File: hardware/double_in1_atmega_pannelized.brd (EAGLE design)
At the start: 82 x 70 mm, 76 parts, among them IC1 MEGA8-AI, IC2 MEGA8-AI, J1 AVR-ISP-6PINAVR-ISP-6PIN-SMAL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, J2 AVR-ISP-6PINAVR-ISP-6PIN-SMAL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

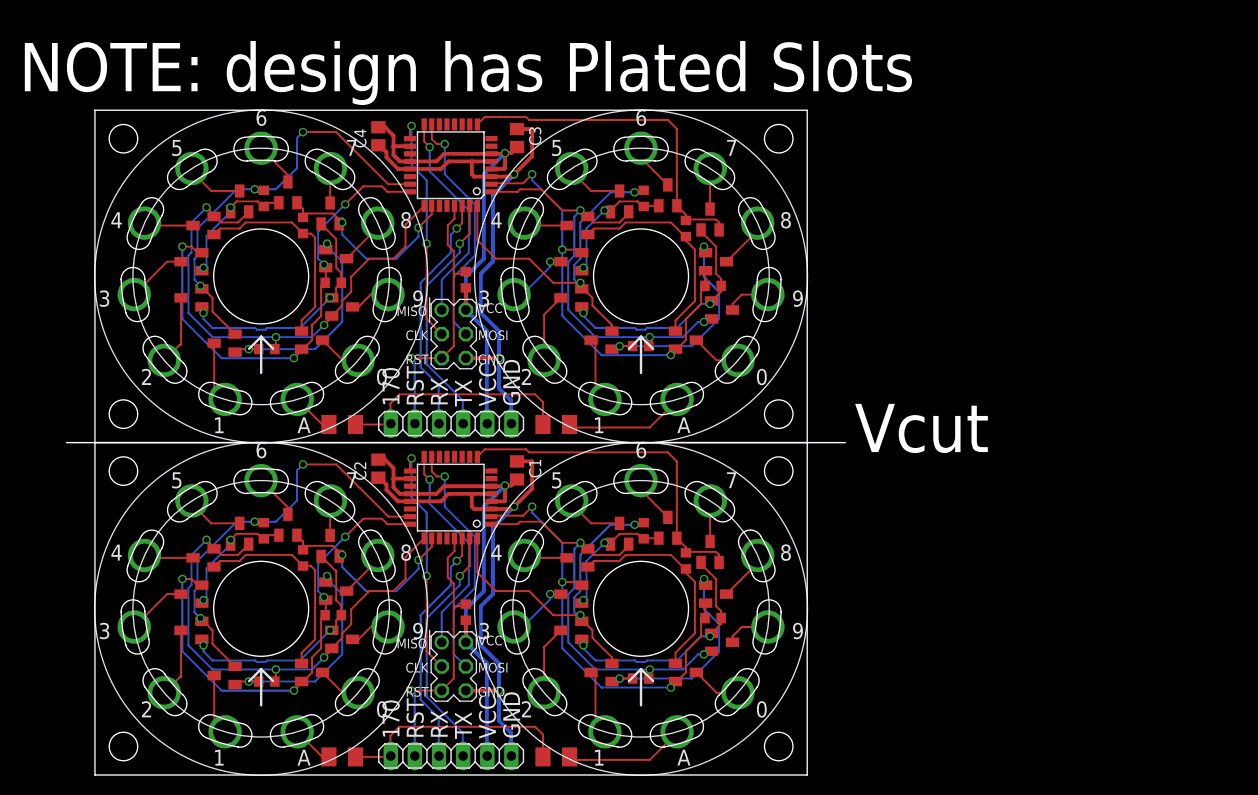
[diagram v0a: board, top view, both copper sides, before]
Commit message: generate gerber for jlpcb
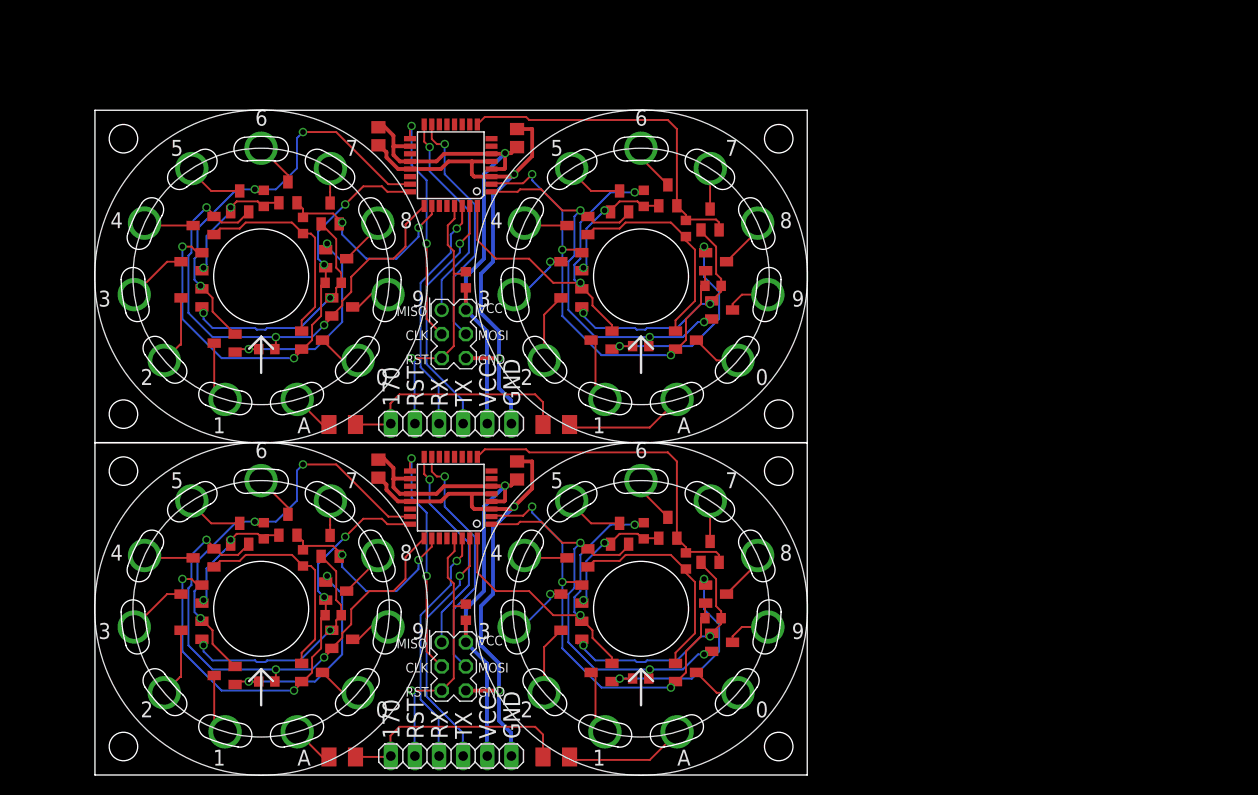
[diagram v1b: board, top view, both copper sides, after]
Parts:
- added GOLD_ORB_SM1, GOLD_ORB_SM2: OSHWLOGOLOGO5MM, oshw:OSHW_5MM
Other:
- board size 82 x 70 mm -> 75 x 70 mm
- board text added: "hackaday.io/project/69708 T Flayols - 2018"
- board text removed: "C1"
- board text removed: "C2"
- board text removed: "NOTE: design has Plated Slots"
- board text removed: "Vcut"
